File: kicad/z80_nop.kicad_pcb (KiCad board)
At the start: 2 copper layers, 82 x 90 mm, 39 parts, among them J1 USB_C_Receptacle_PowerOnly_6P, J2 USB_A, J5 Barrel_Jack, SW1 SW_Push, U1 LM555CN, U2 Z80

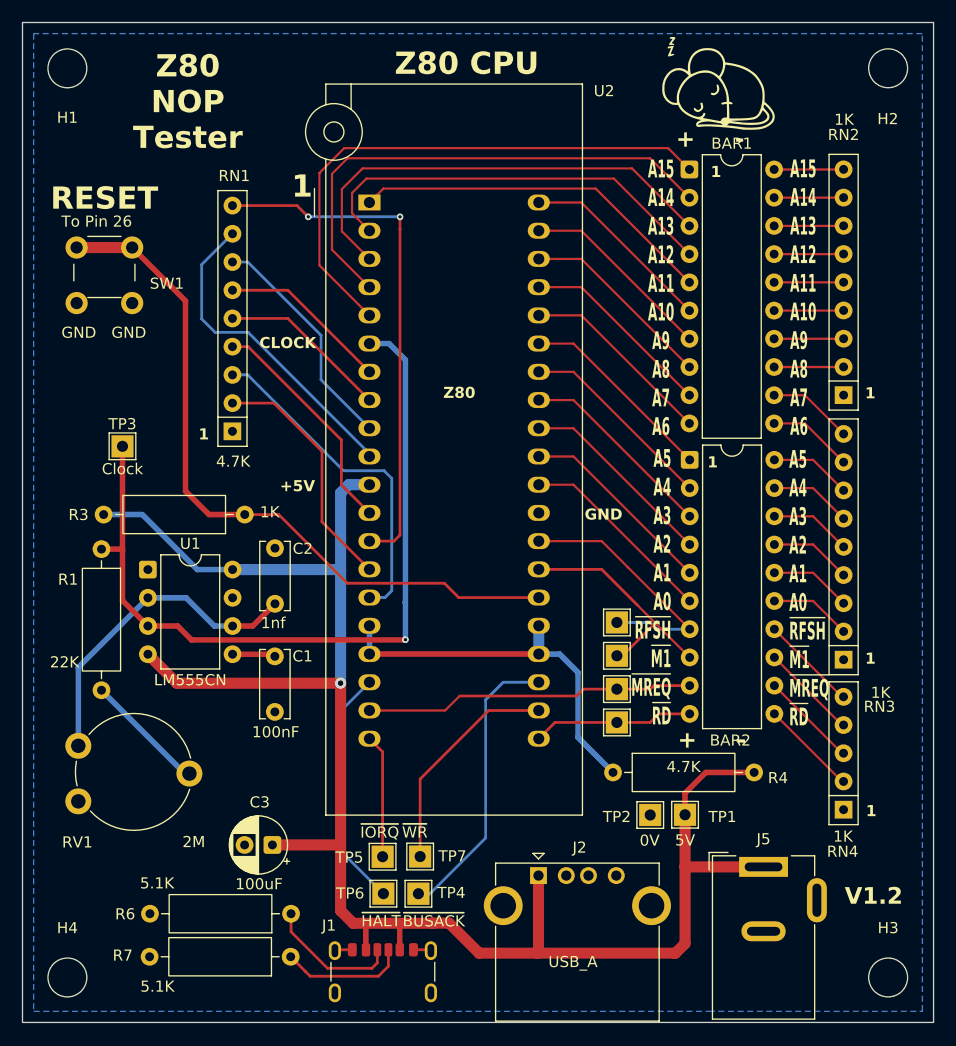
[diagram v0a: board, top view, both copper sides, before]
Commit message: Add HALT mode
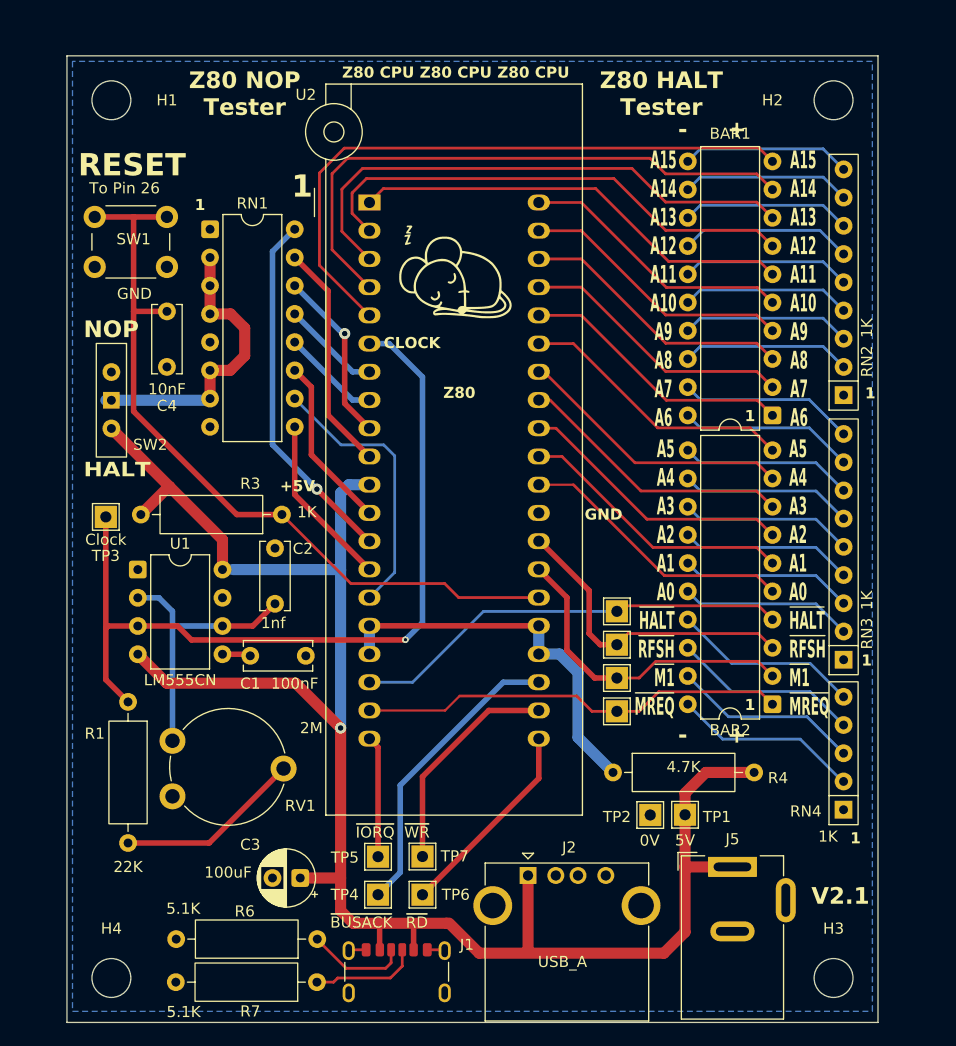
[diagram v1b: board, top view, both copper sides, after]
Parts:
- removed the G001 at (124.5, 113.2)
- added C4: 10nF, Capacitor_THT:C_Disc_D6.0mm_W2.5mm_P5.00mm, F.Cu at (120.0, 131.0)
- added SW2: SW_SPDT, 80_Bus:SW_Slide-03_Pin-2-Common_10x2.5x6.4_P2.54mm, F.Cu at (115.0, 139.0)
- RN1: value 4.7K -> R_Pack08; footprint Resistor_THT:R_Array_SIP9 -> Package_DIP:DIP-16_W7.62mm
- SW1: footprint 80_Bus:SW_PUSH_5mm_H5mm -> Button_Switch_THT:SW_PUSH_6mm_H5mm
- TP6: value ~{HALT} -> ~{RD}
- TP8: value ~{RD} -> ~{HALT}
- moved G002 77.2 mm to (155.0, 188.5)
- moved G001 29.1 mm to (146.0, 127.5)
- moved BAR1 23.4 mm to (174.5, 140.4), turned to 180 degrees
- moved BAR2 23.2 mm to (174.5, 166.4), turned to 180 degrees
- moved RN1 18.3 mm to (123.9, 123.6), turned to 0 degrees
- moved R1 14.0 mm to (116.5, 166.2)
- moved TP8 10.0 mm to (160.5, 158.0)
- moved RV1 8.49 mm to (120.5, 174.7)
- moved TP3 6.53 mm to (114.5, 149.5)
- moved H2 5.70 mm to (180.0, 112.0)
- moved H3 4.91 mm to (180.0, 191.0)
- moved H1 4.89 mm to (115.0, 112.0)
- moved H4 3.96 mm to (115.0, 191.0)
- moved C3 3.89 mm to (132.0, 182.0)
- moved TP4 3.64 mm to (139.0, 183.5)
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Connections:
- BAR1 pad 1: Net-(U2-A15) -> Net-(U2-A6)
- BAR1 pad 10: Net-(U2-A6) -> Net-(U2-A15)
- BAR1 pad 11: Net-(RN3-R7) -> Net-(RN2-R8)
- BAR1 pad 12: Net-(RN3-R8) -> Net-(RN2-R7)
- BAR1 pad 13: Net-(RN2-R1) -> Net-(RN2-R6)
- BAR1 pad 14: Net-(RN2-R2) -> Net-(RN2-R5)
- BAR1 pad 15: Net-(RN2-R3) -> Net-(RN2-R4)
- BAR1 pad 16: Net-(RN2-R4) -> Net-(RN2-R3)
- BAR1 pad 17: Net-(RN2-R5) -> Net-(RN2-R2)
- BAR1 pad 18: Net-(RN2-R6) -> Net-(RN2-R1)
- BAR1 pad 19: Net-(RN2-R7) -> Net-(RN3-R8)
- BAR1 pad 2: Net-(U2-A14) -> Net-(U2-A7)
- BAR1 pad 20: Net-(RN2-R8) -> Net-(RN3-R7)
- BAR1 pad 3: Net-(U2-A13) -> Net-(U2-A8)
- BAR1 pad 4: Net-(U2-A12) -> Net-(U2-A9)
- BAR1 pad 5: Net-(U2-A11) -> Net-(U2-A10)
- BAR1 pad 6: Net-(U2-A10) -> Net-(U2-A11)
- BAR1 pad 7: Net-(U2-A9) -> Net-(U2-A12)
- BAR1 pad 8: Net-(U2-A8) -> Net-(U2-A13)
- BAR1 pad 9: Net-(U2-A7) -> Net-(U2-A14)
- BAR2 pad 1: Net-(U2-A5) -> MREQ
- BAR2 pad 10: RD -> Net-(U2-A5)
- BAR2 pad 11: Net-(RN4-R1) -> Net-(RN3-R6)
- BAR2 pad 12: Net-(RN4-R2) -> Net-(RN3-R5)
- BAR2 pad 13: Net-(RN4-R3) -> Net-(RN3-R4)
- BAR2 pad 14: Net-(RN4-R4) -> Net-(RN3-R3)
- BAR2 pad 15: Net-(RN3-R1) -> Net-(RN3-R2)
- BAR2 pad 16: Net-(RN3-R2) -> Net-(RN3-R1)
- BAR2 pad 17: Net-(RN3-R3) -> Net-(RN4-R4)
- BAR2 pad 18: Net-(RN3-R4) -> Net-(RN4-R3)
- BAR2 pad 19: Net-(RN3-R5) -> Net-(RN4-R2)
- BAR2 pad 2: Net-(U2-A4) -> M1
- BAR2 pad 20: Net-(RN3-R6) -> Net-(RN4-R1)
- BAR2 pad 3: Net-(U2-A3) -> RFSH
- BAR2 pad 4: Net-(U2-A2) -> HALT
- BAR2 pad 5: Net-(U2-A1) -> Net-(U2-A0)
- BAR2 pad 6: Net-(U2-A0) -> Net-(U2-A1)
- BAR2 pad 7: RFSH -> Net-(U2-A2)
- BAR2 pad 8: M1 -> Net-(U2-A3)
- BAR2 pad 9: MREQ -> Net-(U2-A4)
- RN1 pad 2: Net-(RN1-R1) -> Net-(RN1-R2.1)
- RN1 pad 3: Net-(RN1-R2) -> Net-(RN1-R2.1)
- RN1 pad 4: Net-(RN1-R3) -> Net-(RN1-R2.1)
- RN1 pad 5: Net-(RN1-R4) -> GND
- RN1 pad 6: Net-(RN1-R5) -> Net-(RN1-R2.1)
- RN1 pad 7: Net-(RN1-R6) -> Net-(RN1-R2.1)
- RN1 pad 8: Net-(RN1-R7) -> GND
- RN1 pad 9: Net-(RN1-R8) -> Net-(RN1-R8.2)
- TP6 pad 1: Net-(U2-~{HALT}) -> Net-(U2-~{RD})
- TP8 pad 1: RD -> HALT
- U2 pad 10: Net-(RN1-R7) -> Net-(RN1-R2.2)
- U2 pad 12: Net-(RN1-R3) -> Net-(RN1-R6.2)
- U2 pad 13: Net-(RN1-R8) -> Net-(RN1-R1.2)
- U2 pad 14: Net-(RN1-R1) -> Net-(RN1-R8.2)
- U2 pad 15: Net-(RN1-R2) -> Net-(RN1-R7.2)
- U2 pad 18: Net-(U2-~{HALT}) -> HALT
- U2 pad 21: RD -> Net-(U2-~{RD})
- U2 pad 7: Net-(RN1-R5) -> Net-(RN1-R4.2)
- U2 pad 8: Net-(RN1-R4) -> Net-(RN1-R5.2)
- U2 pad 9: Net-(RN1-R6) -> Net-(RN1-R3.2)
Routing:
- net Net-(RN1-R8): track 47.1 -> 0.00 mm, vias 2 -> 0
- net HALT: track 0.00 -> 39.6 mm
- net Net-(RN1-R1.2): track 0.00 -> 32.5 mm, vias 0 -> 1
- net Net-(RN1-R2): track 30.6 -> 0.00 mm
- net Net-(RN1-R7): track 28.9 -> 0.00 mm
- net Net-(RN1-R2.1): track 0.00 -> 26.9 mm
- net Net-(RN1-R7.2): track 0.00 -> 24.8 mm
- net Net-(RN1-R1): track 22.3 -> 0.00 mm
- net Net-(U2-~{HALT}): track 21.5 -> 0.00 mm
- net Net-(RN1-R3): track 20.9 -> 0.00 mm
- net Net-(RN1-R6): track 20.9 -> 0.00 mm
- net Net-(RN1-R2.2): track 0.00 -> 20.7 mm
- net Net-(U2-~{RD}): track 0.00 -> 18.4 mm
- net Net-(RN1-R3.2): track 0.00 -> 15.7 mm, vias 0 -> 1
- net Net-(RN1-R8.2): track 0.00 -> 15.6 mm
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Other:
- board size 82 x 90 mm -> 73 x 87 mm
- board text added: "- +"
- board text added: "31a058fe-c457-4991-a0f4-a968bf82c0ea"
- board text added: "A5 A4 A3 A2 A1 A0 ~{HALT} ~{RFSH} ~{M1} ~{MREQ}"
- board text added: "HALT"
- board text added: "NOP"
- board text added: "V2.1"
- board text added: "Z80 CPU Z80 CPU Z80 CPU"
- board text added: "Z80 HALT Tester"
- board text removed: "+ -"
- board text removed: "9e66cd35-b514-4867-88cf-f9ff6f002000"
- board text removed: "A5 A4 A3 A2 A1 A0 ~{RFSH} ~{M1} ~{MREQ} ~{RD}"
- board text removed: "V1.2"
- board text removed: "Z80 CPU"
